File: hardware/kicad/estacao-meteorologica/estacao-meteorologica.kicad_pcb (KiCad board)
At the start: 2 copper layers, 109.4 x 61.3 mm, 125 parts, among them J101 Header, 1x02, P2.54 mm, J102 Header, 1x06, P2.54 mm, J103 Header, 1x03, P2.54 mm, J221 JST-XH, 1x04, P2.50 mm, J301 RJ11 6P6C, 90°, J501 RJ11 6P6C, 90°, J601 DC jack, 2.0 mm, J602 JST-XH, 1x02, P2.50 mm, J701 U.FL, 50 Ω, J801 microSD socket, TF-15x15, Q601 DMP6023LE-13, SW101 Tactile switch, SPST, U101 STM32F446RET6, U211 BMP280, U231 DHT22, U301 SN74LVC1G17DBVR, U401 SN74LVC1G17DBVR, U601 AP63203WU-7, U701 LORA1276-C1-915MHZ, U801 SN74LVC125APWR, U802 EMIF06-MSD02N16, Y101 32.768 kHz, CL 7 pF, Y102 8 MHz, CL 10 pF

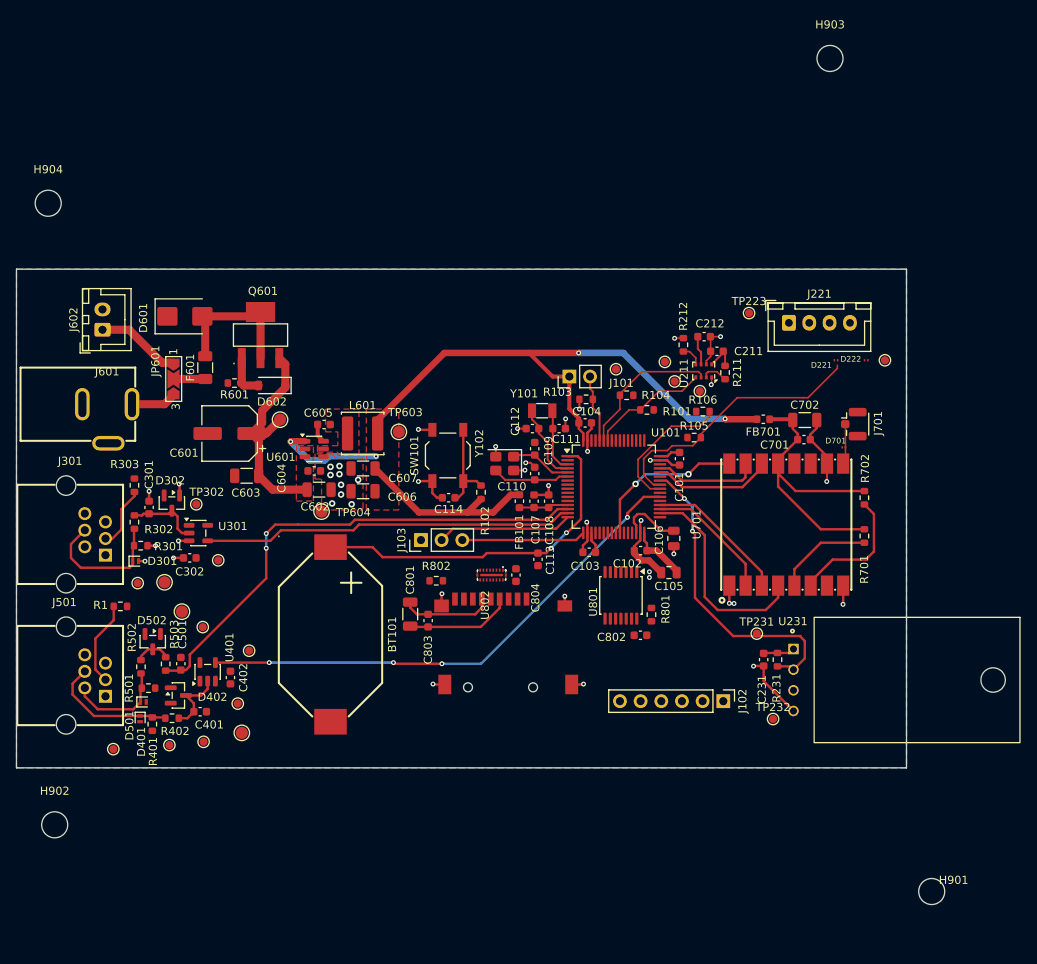
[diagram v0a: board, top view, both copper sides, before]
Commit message: feat(hardware): consolida revisão PCB V2
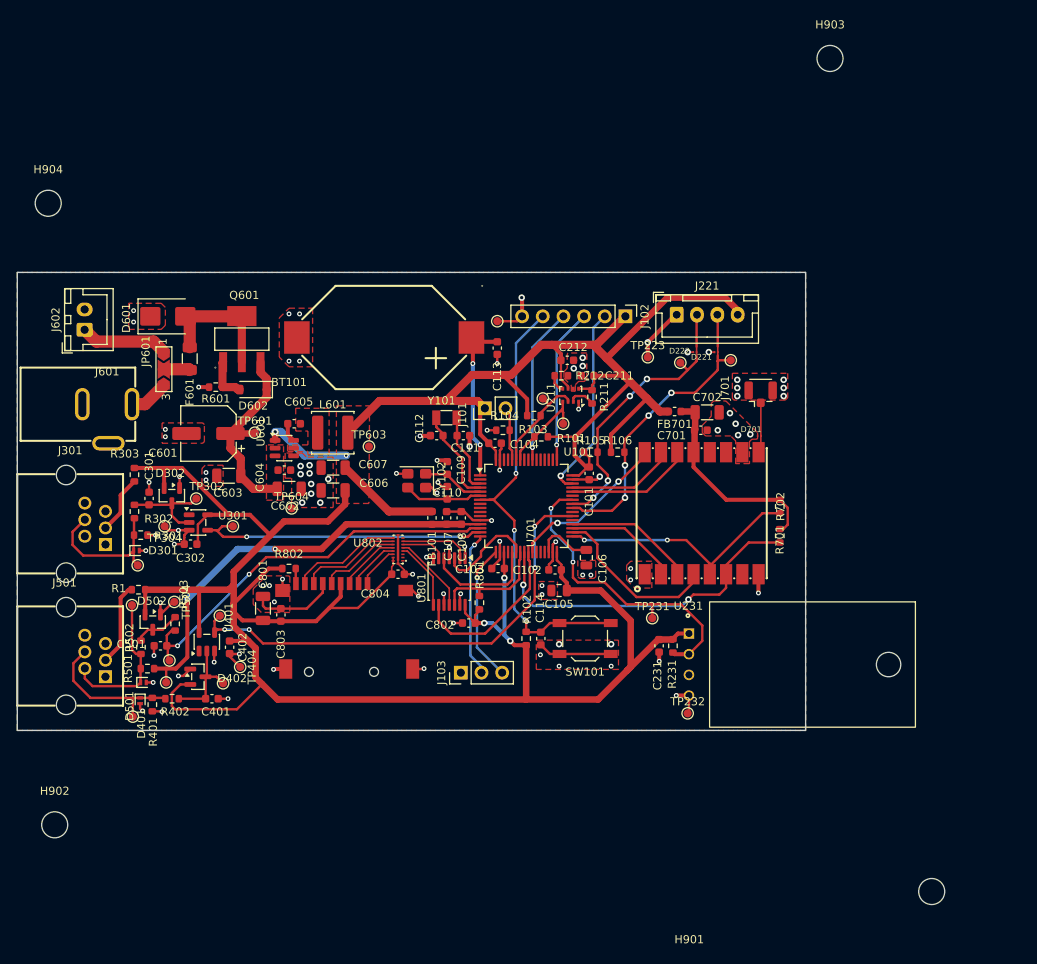
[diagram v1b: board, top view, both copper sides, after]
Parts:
- TP304, TP404, TP504, TP601, TP603, TP604: footprint TestPoint:TestPoint_Pad_D1.5mm -> TestPoint:TestPoint_Pad_D1.0mm
- moved J102 48.8 mm to (113.2, 57.8)
- moved BT101 37.1 mm to (83.6, 60.4), turned to 180 degrees
- moved SW101 28.1 mm to (108.3, 97.4), turned to 0 degrees
- moved C113 26.5 mm to (97.5, 61.7)
- moved TP213 26.3 mm to (97.5, 58.4)
- moved TP222 25.2 mm to (120.0, 63.5)
- moved R801 21.2 mm to (95.3, 93.0)
- moved U801 21.2 mm to (91.6, 90.4)
- moved C802 21.2 mm to (94.0, 95.5)
- moved D222 21.1 mm to (121.8, 62.2)
- moved C114 20.7 mm to (102.8, 97.4), turned to -90 degrees
- moved J801 19.6 mm to (79.1, 95.9)
- moved R102 18.8 mm to (101.0, 97.4)
- moved R802 18.2 mm to (71.9, 88.8)
- moved C801 18.1 mm to (68.7, 93.7)
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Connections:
- D221 pad 2: /BH1750_INTERFACE/BH_I2C3_SCL -> /BH1750_INTERFACE/BH_I2C3_SDA
- D222 pad 2: /BH1750_INTERFACE/BH_I2C3_SDA -> /BH1750_INTERFACE/BH_I2C3_SCL
- J102 pad 2: GND -> SWDIO
- J102 pad 3: SWDIO -> SWCLK
- J102 pad 4: SWCLK -> SWO
- J102 pad 6: SWO -> GND
- J221 pad 2: /BH1750_INTERFACE/BH_I2C3_SDA -> /BH1750_INTERFACE/BH_I2C3_SCL
- J221 pad 3: /BH1750_INTERFACE/BH_I2C3_SCL -> /BH1750_INTERFACE/BH_I2C3_SDA
- J221 pad 4: unconnected-(J221-Pin_4-Pad4) -> +3V3
- R801 pad 1: /CARTÃO microSD/SD_SPI_CS -> /CARTÃO microSD/SD_SPI_MOSI
- TP221 pad 1: /BH1750_INTERFACE/BH_I2C3_SCL -> /BH1750_INTERFACE/BH_I2C3_SDA
- TP222 pad 1: /BH1750_INTERFACE/BH_I2C3_SDA -> /BH1750_INTERFACE/BH_I2C3_SCL
- U801 pad 11: SD_CS_BUF -> SD_MOSI_BUF
- U801 pad 12: /CARTÃO microSD/SD_SPI_CS -> /CARTÃO microSD/SD_SPI_MOSI
- U801 pad 2: /CARTÃO microSD/SD_SPI_MOSI -> SD_MISO_BUF
- U801 pad 3: SD_MOSI_BUF -> /CARTÃO microSD/SD_MISO
- U801 pad 5: SD_MISO_BUF -> /CARTÃO microSD/SD_SCK
- U801 pad 6: /CARTÃO microSD/SD_MISO -> SD_SCK_BUF
- U801 pad 8: SD_SCK_BUF -> SD_CS_BUF
- U801 pad 9: /CARTÃO microSD/SD_SCK -> /CARTÃO microSD/SD_SPI_CS
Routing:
- net +3V3: track 143.6 -> 404.9 mm, vias 4 -> 5
- net AVREF_SENSOR: track 6.06 -> 53.3 mm, vias 0 -> 2
- net NRST: track 11.4 -> 56.1 mm, vias 0 -> 3
- net GND: track 90.5 -> 121.3 mm, vias 43 -> 95
- net /MCU E DEPURAÇÃO/LORA_RST: track 16.1 -> 42.4 mm, vias 0 -> 2
- net SWDIO: track 0.00 -> 23.9 mm, vias 0 -> 1
- net VBAT: track 42.4 -> 20.8 mm
- net /BH1750_INTERFACE/BH_I2C3_SDA: track 17.0 -> 37.9 mm, vias 0 -> 4
- net /CARTÃO microSD/SD_SPI_CS: track 0.00 -> 20.7 mm
- net /MCU E DEPURAÇÃO/LORA_NSS: track 12.0 -> 31.9 mm, vias 0 -> 2
- net SWO: track 0.00 -> 19.2 mm, vias 0 -> 1
- net SWCLK: track 0.00 -> 19.0 mm, vias 0 -> 1
- net /CARTÃO microSD/SD_SPI_MOSI: track 0.00 -> 14.6 mm
- net /CARTÃO microSD/SD_SCK: track 0.00 -> 14.1 mm
- net SD_CARD_DAT1: track 0.00 -> 13.8 mm
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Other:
- board size 109.4 x 61.3 mm -> 96.9 x 56.3 mm
